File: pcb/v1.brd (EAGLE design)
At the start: 92 x 80 mm, 61 parts, among them T1 MMBT3904, T2 MMBT3904, T3 MMBT3904, T4 MMBT3904

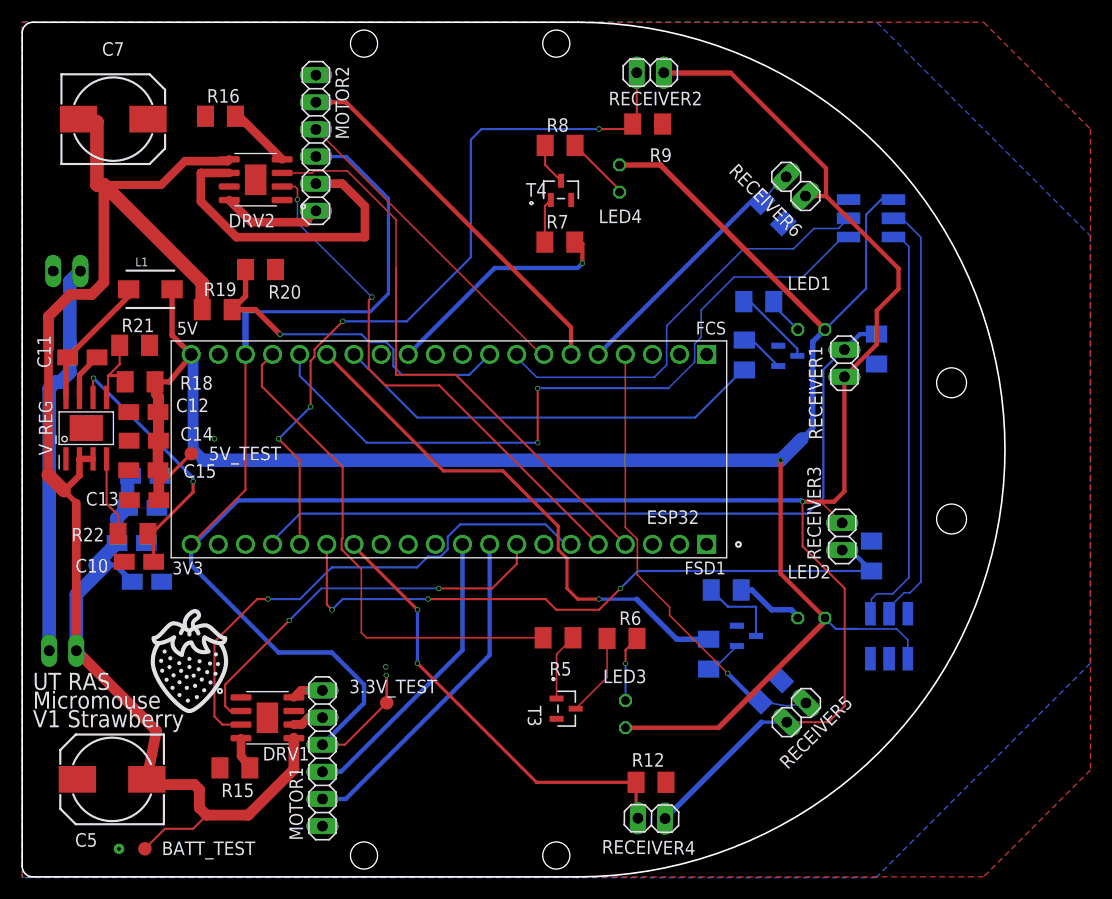
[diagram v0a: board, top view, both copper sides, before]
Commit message: Changed PCB
Fixes #11
Fixes #10
Fixes #9
Fixes #8
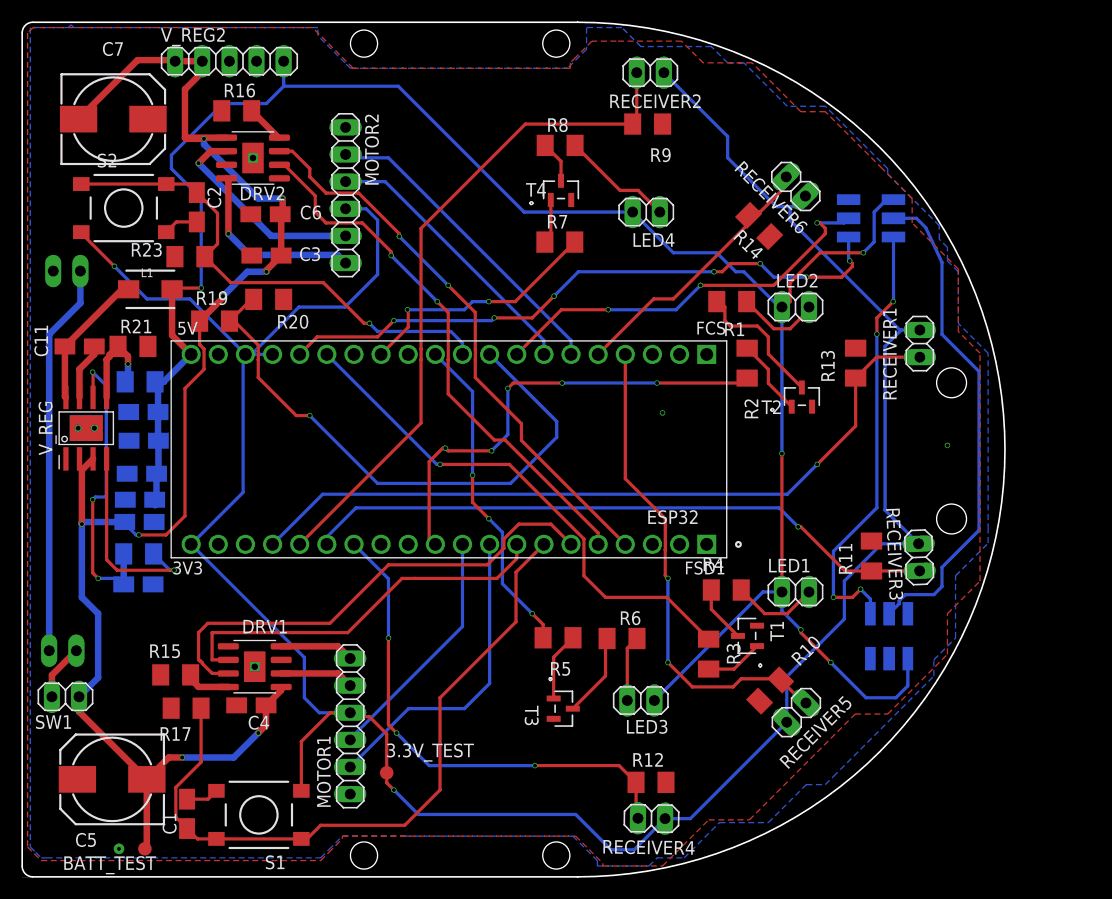
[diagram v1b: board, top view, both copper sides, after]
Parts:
- removed 5V_TEST: PTR1B1,27, testpad:B1,27
- added C1, C2: 10uF, rcl:A/3216-18R
- added R17, R23: 10k, rcl:M1206
- added S1, S2: DTSM-6, switch-tact:DTSM-6
- added SW1: (no value), pinhead:1X02
- added V_REG2: (no value), pinhead:1X05
- C12, C13, C14, C15: value 10uF -> 22uF
- LED1, LED2, LED3, LED4: device led:LED5MM -> pinhead:1X02
- moved C6 36.1 mm to (22.8, 62.0), flipped to the top
- moved LED2 29.1 mm to (72.4, 53.3), turned to 0 degrees
- moved LED1 24.6 mm to (72.4, 26.7), turned to 0 degrees
- moved C3 23.5 mm to (22.9, 58.2), flipped to the top
- moved C4 18.9 mm to (21.5, 16.1), flipped to the top
- moved R15 10.3 mm to (14.4, 18.9)
- moved RECEIVER3 7.46 mm to (84.0, 29.9), turned to 272.2 degrees
- moved RECEIVER1 7.30 mm to (84.0, 49.9), turned to 270 degrees
- moved 3.3V_TEST 6.55 mm to (34.1, 9.74)
- moved MOTOR2 5.62 mm to (30.3, 63.8)
- moved DRV1 4.93 mm to (21.8, 19.7)
- moved T2 4.02 mm to (73.0, 45.0), flipped to the top, turned to 0 degrees
- moved LED4 4.01 mm to (58.4, 62.2), turned to 0 degrees
- moved MOTOR1 3.96 mm to (30.7, 14.1)
- moved R20 2.90 mm to (23.1, 54.1)
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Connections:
- removed net N$11: LED3.K, R6.2
- new net LED3: LED3.2, R6.2
- new net N$22: C2.+, S2.4
- new net N$3: BATT1.1, SW1.1
- new net N$4: C1.+, S1.4
- new net SW1: C1.-, ESP32.J2_7, R17.2, S1.1, S1.2
- new net SW2: C2.-, ESP32.J3_10, R23.2, S2.1, S2.2
- net 3.3V: now also ESP32.J3_17, S1.3, S2.3
- net 5V: now also LED1.1, LED2.1, LED3.1, LED4.1, V_REG2.5; no longer 5V_TEST.TP, LED1.A, LED2.A, LED3.A, LED4.A
- net BATT_POWER: now also SW1.2, V_REG2.1, V_REG2.2; no longer BATT1.1
- net EM1: now also ESP32.J2_11; no longer ESP32.J3_14
- net EM3: now also ESP32.J3_11; no longer ESP32.J3_17
- net EM4: now also ESP32.J3_13; no longer ESP32.J3_12
- net GND: now also DRV1.P$1, DRV2.P$1, R17.1, R23.1, V_REG.P$1, V_REG.P$2, V_REG2.3, V_REG2.4
- net N$14: now also LED4.2; no longer LED4.K
- net N$6: now also LED2.2; no longer LED1.K
- net N$8: now also LED1.2; no longer LED2.K
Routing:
- net SW1: track 0.00 -> 65.7 mm
- net SW2: track 0.00 -> 47.0 mm, vias 0 -> 1
- net 3.3V: track 261.3 -> 238.2 mm
- net V_SENSE: track 32.6 -> 54.0 mm
- net EM3: track 47.6 -> 30.7 mm, vias 0 -> 3
- net BATT_POWER: track 156.2 -> 143.2 mm, vias 0 -> 8
- net PG: track 7.44 -> 18.7 mm, vias 0 -> 1
- net N$19: track 30.4 -> 19.7 mm, vias 0 -> 1
- net LED_SIG: track 69.4 -> 59.1 mm, vias 2 -> 7
- net 5V: track 199.6 -> 190.9 mm, vias 1 -> 5
- net N$18: track 9.56 -> 17.4 mm, vias 0 -> 1
- net REC2: track 70.4 -> 63.1 mm, vias 4 -> 0
- net N$11: track 6.26 -> 0.00 mm
- net N$34: track 40.1 -> 46.4 mm
- net LED3: track 0.00 -> 6.18 mm
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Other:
- board text removed: "Micromouse"
- board text removed: "UT RAS"
- board text removed: "V1 Strawberry"

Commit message: Cosmetic Changes
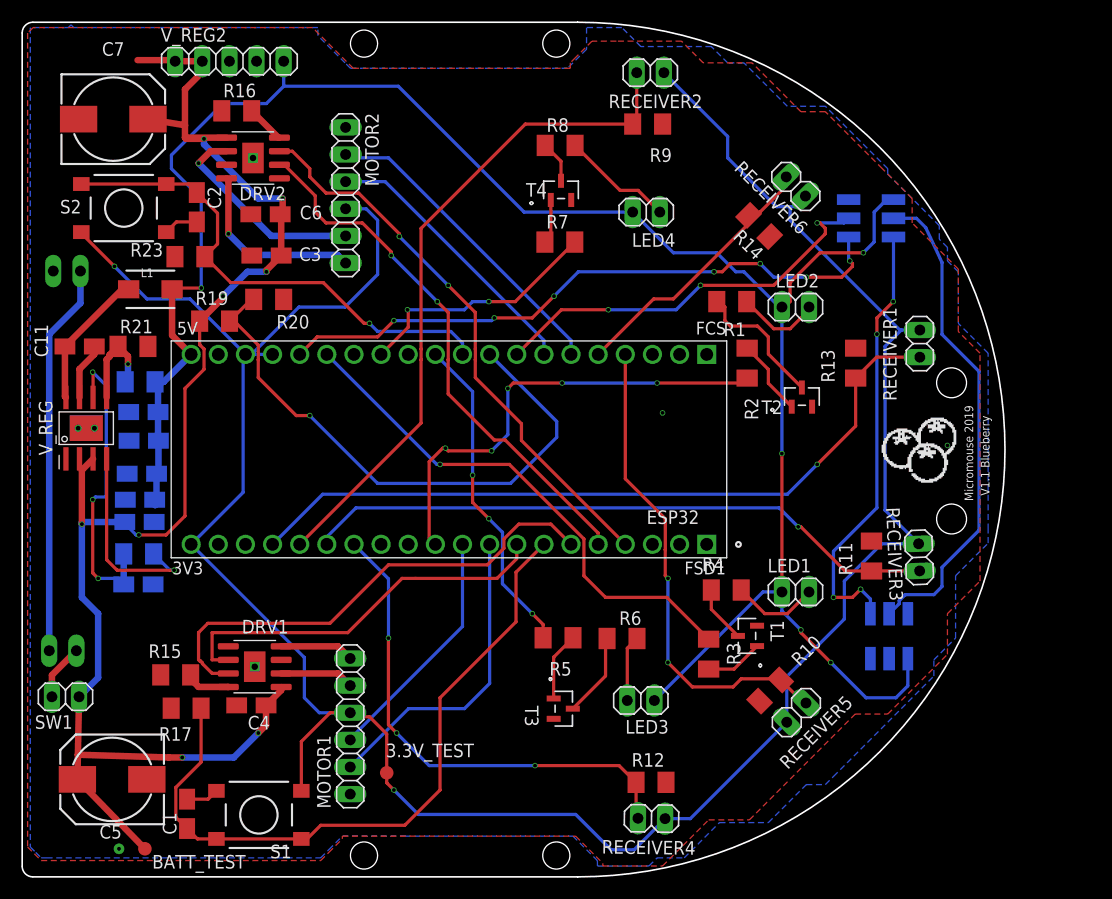
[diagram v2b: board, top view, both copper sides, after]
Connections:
- net BATT_POWER: now also C5.+, C7.+; no longer C5.-, C7.-
- net GND: now also C5.-, C7.-; no longer C5.+, C7.+
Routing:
- net BATT_POWER: track 143.2 -> 146.0 mm
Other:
- board text added: "Micromouse 2019"
- board text added: "V1.1 Blueberry"
- board text removed: "/Users/vamsighorakavi/Downloads/strawberry(2).bmp"
